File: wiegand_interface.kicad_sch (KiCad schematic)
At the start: 10 parts, among them U7 LTV-827S, U8 LTV-827S

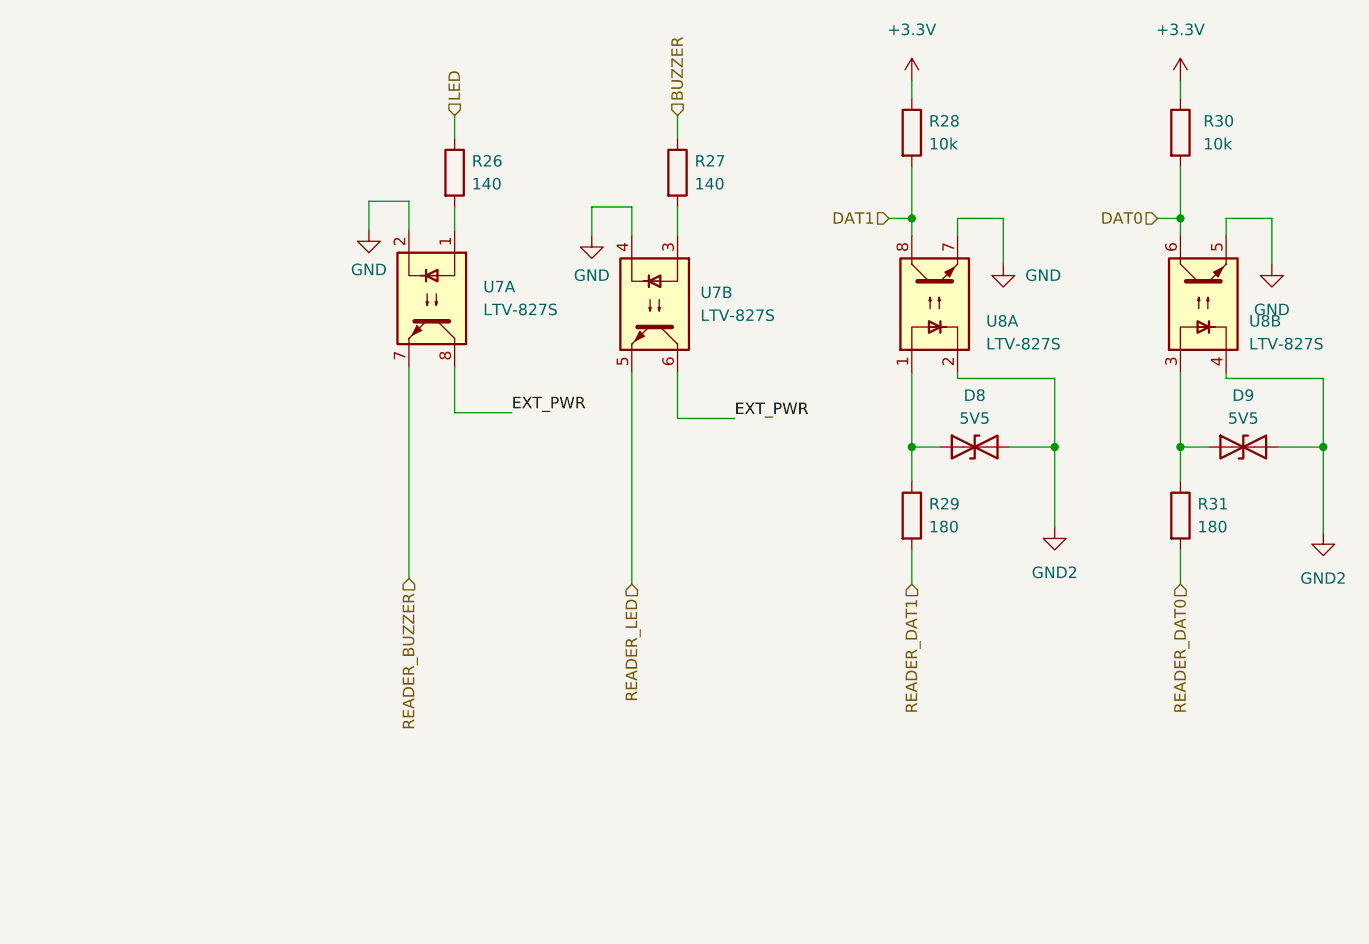
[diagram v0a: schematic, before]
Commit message: DO the bulk of rev 1.2 layout
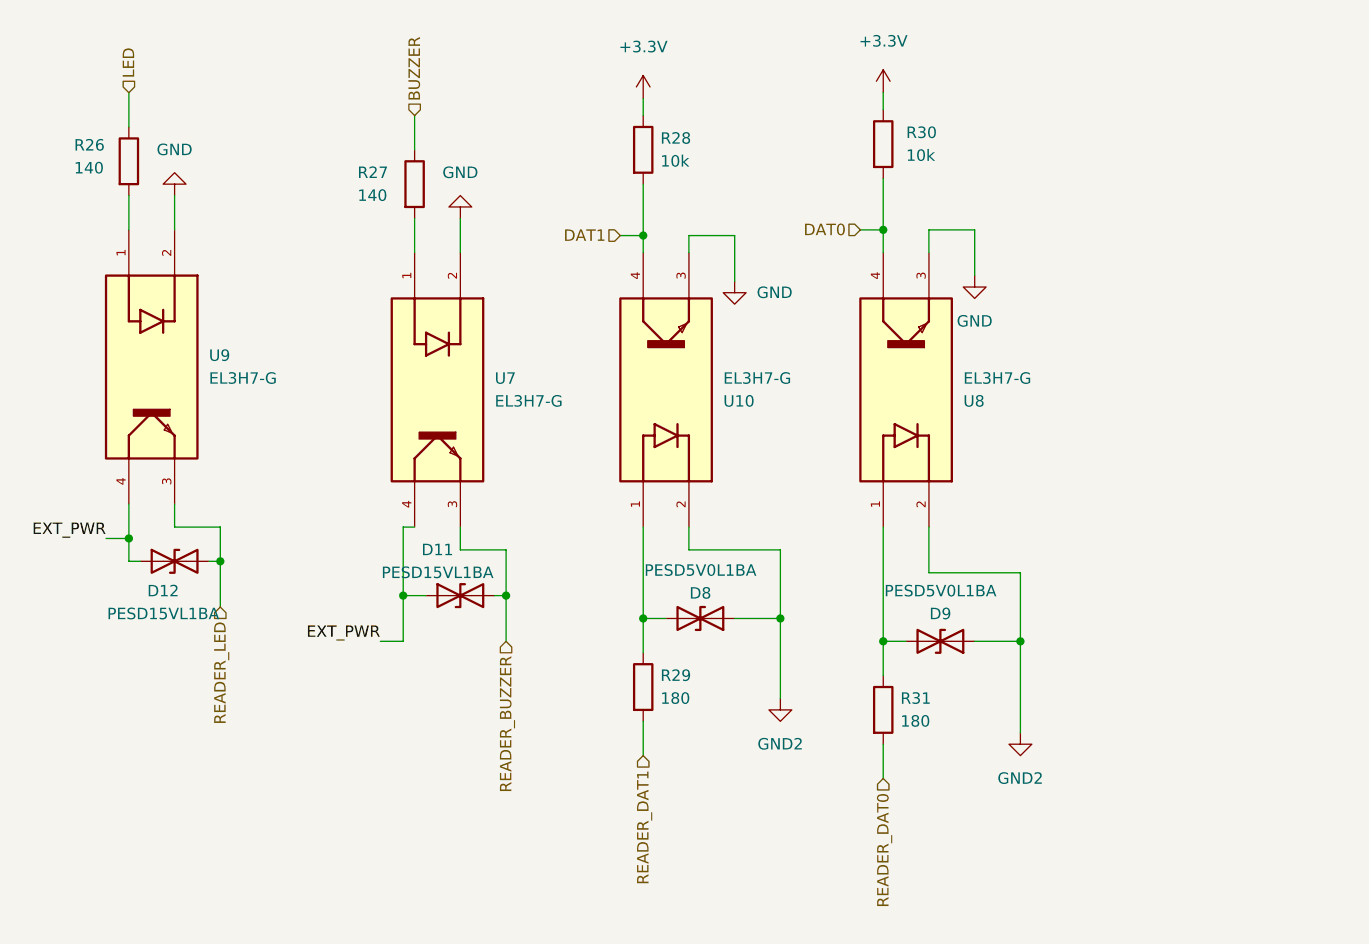
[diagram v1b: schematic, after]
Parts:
- removed U7, U8: LTV-827S, Package_DIP:SMDIP-8_W9.53mm, symbol Isolator:LTV-827S
- added D11, D12: PESD15VL1BA, Diode_SMD:D_SOD-323, symbol Device:D_TVS
- added U10, U7, U8, U9: EL3H7-G, project specific:SOIC127P700X200-4N, symbol EL3H7-G:EL3H7-G
- D8, D9: value 5V5 -> PESD5V0L1BA; footprint Diode_SMD:D_SMA-SMB_Universal_Handsoldering -> Diode_SMD:D_SOD-323; LCSC (none) -> C85380
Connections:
- net DAT0: now also U8.4
- net DAT1: now also U10.4
- net EXT_PWR: now also D11.1 (A1), D12.1 (A1), U7.4, U9.4
- net GND: now also U10.3, U7.2, U8.3, U9.2
- net GND2: now also D8.1 (A1), D9.1 (A1), U10.2, U8.2; no longer D8.2 (A2), D9.2 (A2)
- net READER_BUZZER: now also D11.2 (A2), U7.3
- net READER_LED: now also D12.2 (A2), U9.3
- net at R26.2: now also U9.1
- net at R27.2: now also U7.1
- net at R29.1: now also D8.2 (A2), U10.1; no longer D8.1 (A1)
- net at R31.1: now also D9.2 (A2), U8.1; no longer D9.1 (A1)
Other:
- moved on the sheet: D8, R26, R27, R28, R29, R30, R31
